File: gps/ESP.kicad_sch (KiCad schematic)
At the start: 18 parts, among them J12 ENC+RGB, J13 ENC+RGB, J7 USB_B_Micro, J9 USB_pads, SW1 RotaryEncoder_Switch, U3 DFR0654

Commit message: PCB-update
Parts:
- SW1: footprint Rotary_Encoder:RotaryEncoder_Alps_EC12E-Switch_Vertical_H20mm_CircularMountingHoles -> Rotary_Encoder:RotaryEncoder_20mm_WO_mount_holes
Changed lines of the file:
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@@
 			)
 		)
-		(property "Footprint" "Rotary_Encoder:RotaryEncoder_Alps_EC12E-Switch_Vertical_H20mm_CircularMountingHoles"
+		(property "Footprint" "Rotary_Encoder:RotaryEncoder_20mm_WO_mount_holes"
 			(at 44.45 41.656 0)
 			(effects

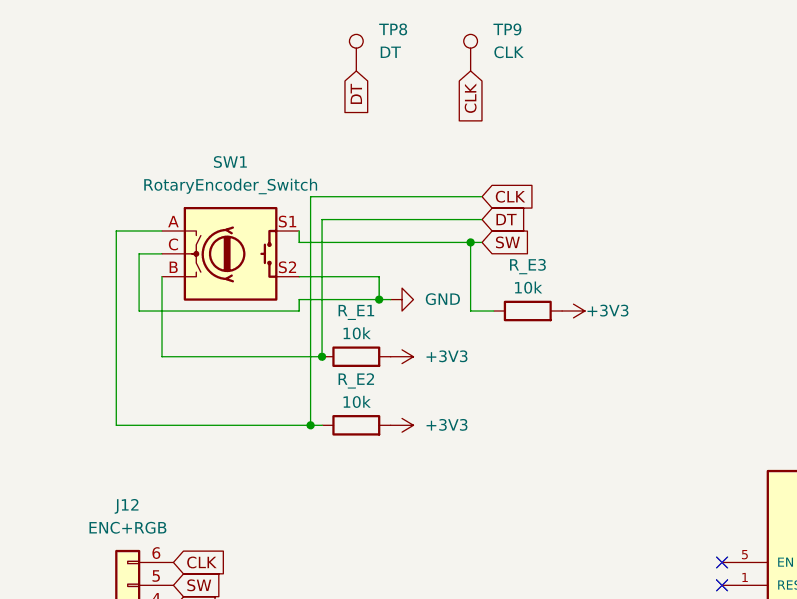
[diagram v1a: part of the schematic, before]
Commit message: tweaks
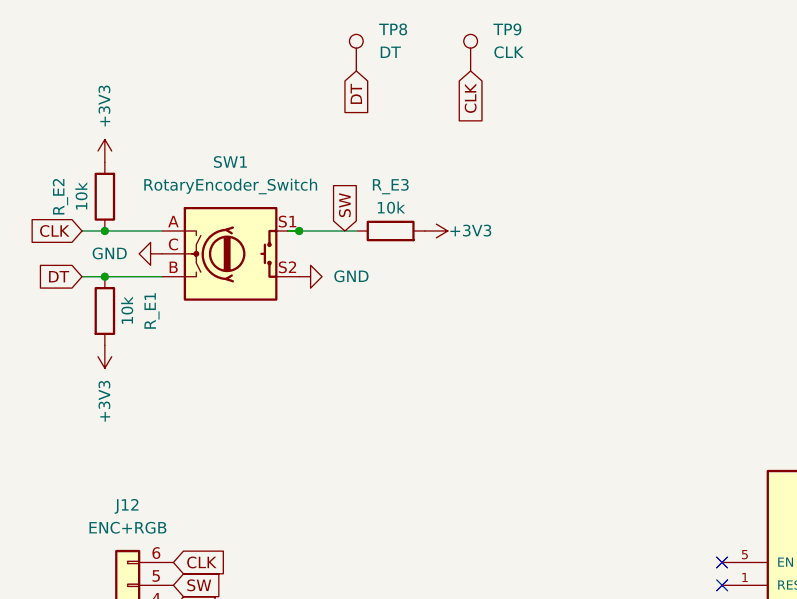
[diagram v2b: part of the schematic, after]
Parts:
- J7: footprint Connector_USB:USB_Mini-B_Tensility_54-00023_Vertical_CircularHoles -> KiCad:USB3145301A
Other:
- moved on the sheet: R_E1, R_E2, R_E3
